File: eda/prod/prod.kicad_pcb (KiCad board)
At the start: 2 copper layers, 58 parts, among them IC1 IC_CH552G, J1 USB_B_Micro, J2 Conn_01x02, SW1 SPDT_C136659, SW2 TS2306A

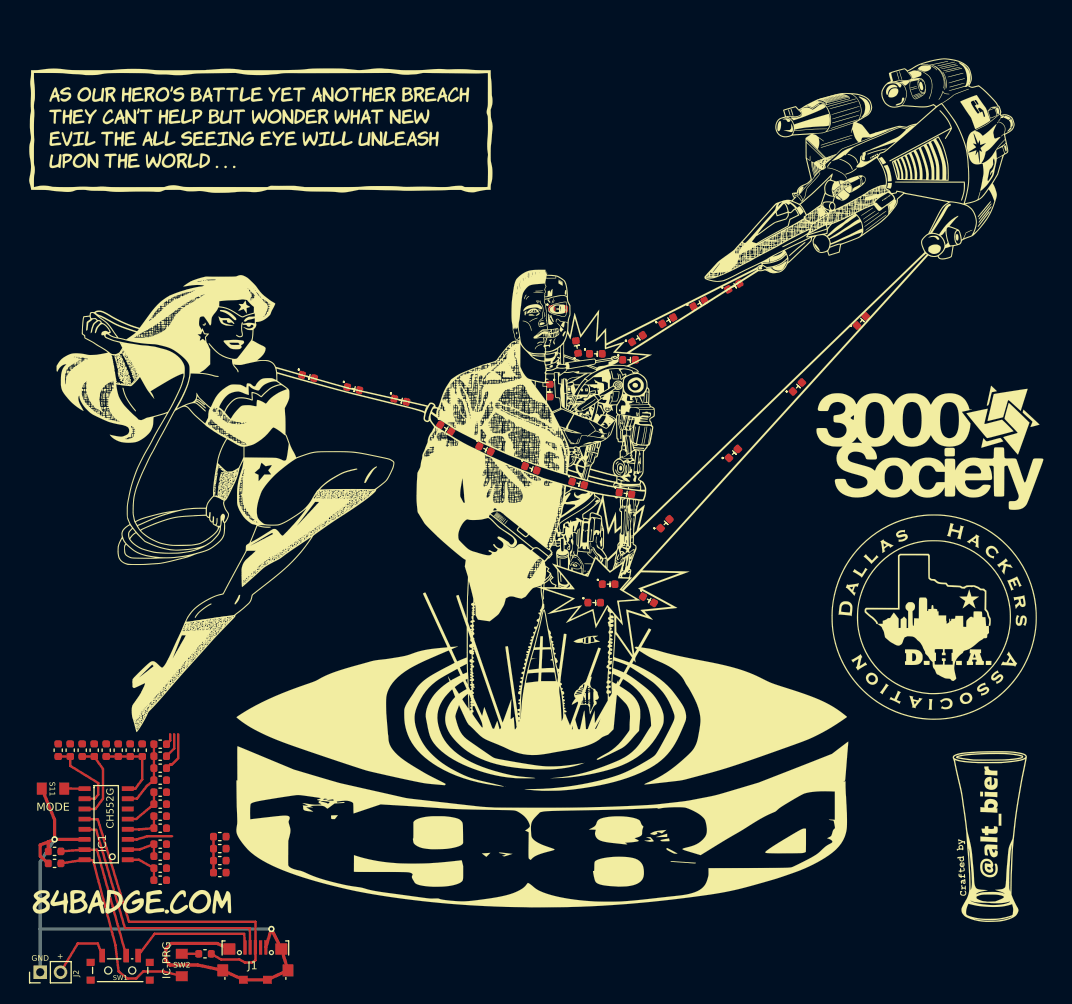
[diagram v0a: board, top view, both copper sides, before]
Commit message: More PCB Layout work
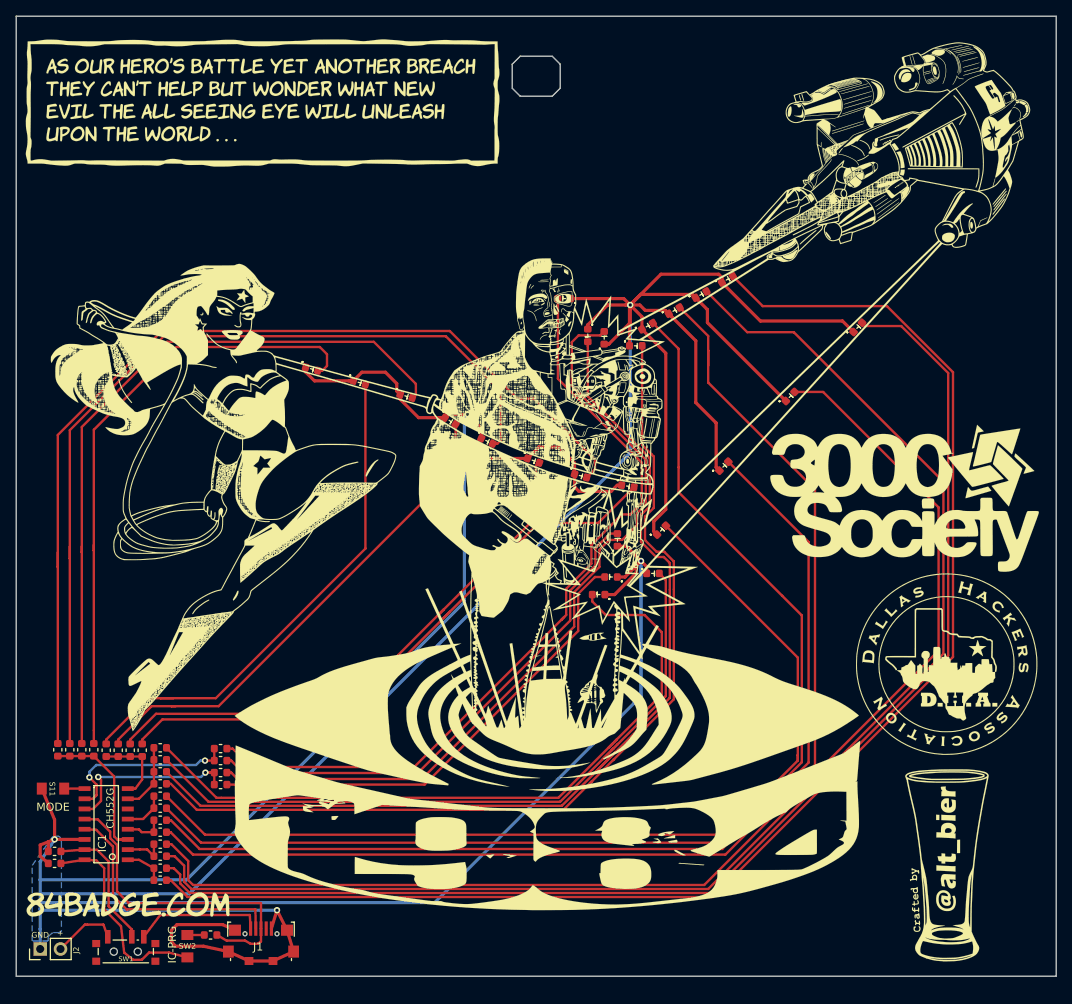
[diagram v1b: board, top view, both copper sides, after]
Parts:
- removed the G*** at (142.0, 83.2)
- added G***: LOGO, 0_local:84_Badge_Silk_900dpi_127mm, F.Cu at (141.5, 84.5)
- moved D322 34.4 mm to (182.2, 62.9), turned to 47 degrees
- moved R154 23.0 mm to (82.2, 115.7), turned to 90 degrees
- moved R153 22.5 mm to (83.7, 115.7), turned to 90 degrees
- moved R152 22.1 mm to (85.2, 115.7), turned to 90 degrees
- moved R151 22.0 mm to (86.7, 115.7), turned to 90 degrees
- moved D332 20.5 mm to (152.2, 89.5), turned to 90 degrees
- moved R332 20.3 mm to (102.5, 117.0), turned to 0 degrees
- moved R331 18.8 mm to (102.5, 115.5), turned to 0 degrees
- moved R341 17.5 mm to (102.5, 118.5), turned to 0 degrees
- moved R342 16.4 mm to (102.5, 120.0), turned to 0 degrees
- moved D162 13.5 mm to (165.5, 80.2)
- moved D321 13.5 mm to (165.9, 56.9), turned to 30 degrees
- moved D172 13.1 mm to (157.7, 88.2)
- moved D142 13.0 mm to (173.7, 71.5)
- moved D313 8.21 mm to (156.6, 93.7)
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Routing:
- net GND: track 96.2 -> 617.8 mm, vias 2 -> 5
- net Net-(D321-Pad2): track 0.00 -> 179.7 mm
- net Net-(D141-Pad2): track 0.00 -> 173.1 mm
- net Net-(D322-Pad2): track 0.00 -> 160.6 mm
- net Net-(D142-Pad2): track 0.00 -> 154.0 mm
- net Net-(D161-Pad2): track 0.00 -> 153.0 mm
- net Net-(D171-Pad2): track 0.00 -> 148.0 mm
- net Net-(D162-Pad2): track 0.00 -> 128.0 mm
- net Net-(D154-Pad2): track 0.00 -> 122.3 mm
- net Net-(D172-Pad2): track 0.00 -> 121.5 mm
- net Net-(D312-Pad2): track 4.98 -> 124.1 mm
- net Net-(D311-Pad2): track 0.00 -> 118.4 mm
- net Net-(D153-Pad2): track 0.00 -> 109.5 mm
- net Net-(D331-Pad2): track 0.00 -> 101.1 mm
- net Net-(D341-Pad2): track 0.00 -> 100.3 mm
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- added copper zone on B.Cu, net GND
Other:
- board outline added: 130 x 120 mm
